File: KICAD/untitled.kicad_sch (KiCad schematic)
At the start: 46 parts, among them IC1 TPA3116D2QDADRQ1, U5 LM321

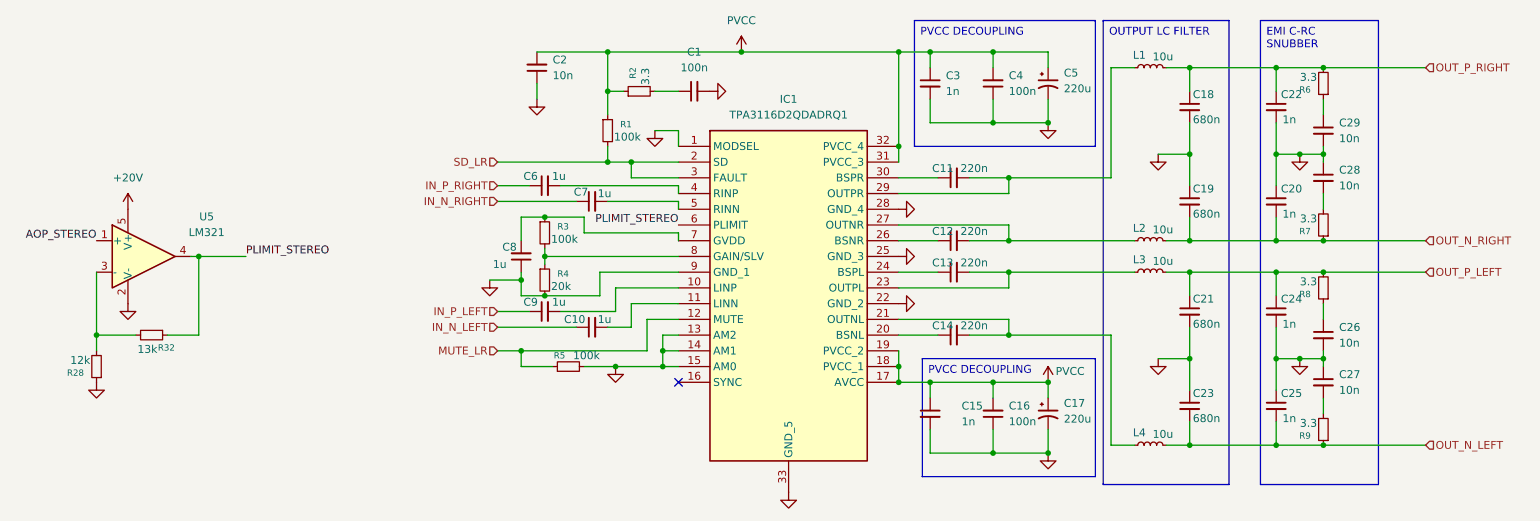
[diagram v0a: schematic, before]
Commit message: mise en forme globale
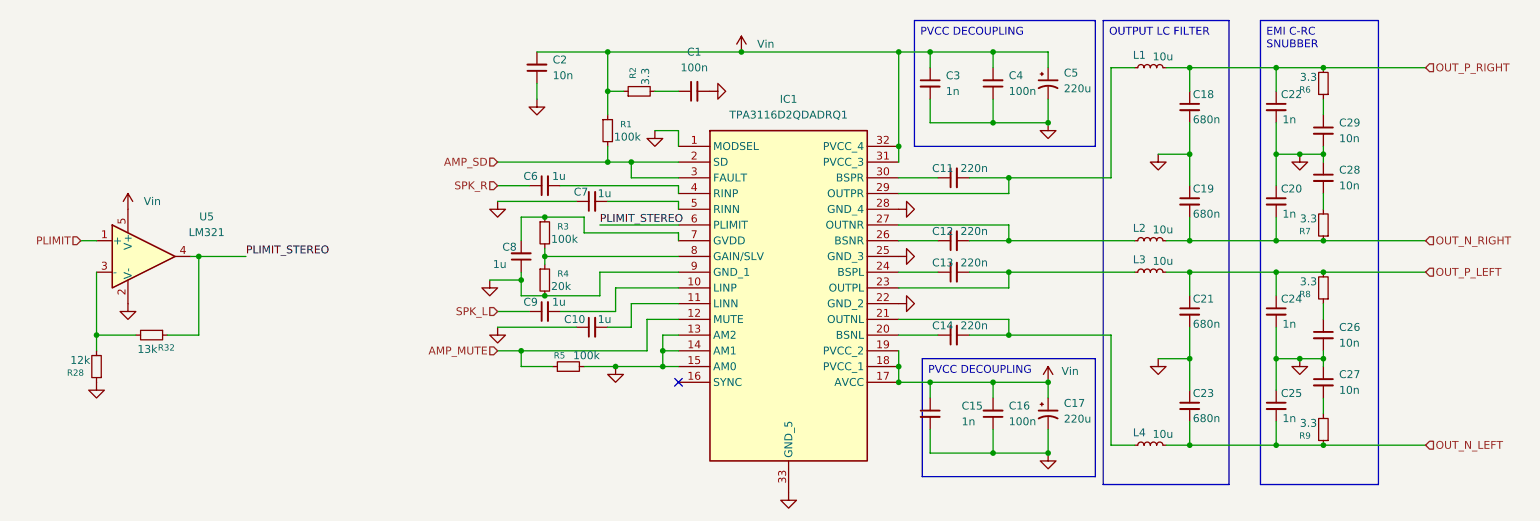
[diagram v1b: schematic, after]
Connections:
- net IN_N_LEFT is gone; now on net GND: C10.1
- net IN_N_RIGHT is gone; now on net GND: C7.1
- net PVCC is gone; now on net Vin: C15.1, C16.2, C17.1, C2.2, C3.1, C4.2, C5.1, IC1.17 (AVCC), IC1.18 (PVCC_1), IC1.19 (PVCC_2), IC1.31 (PVCC_3), IC1.32 (PVCC_4), R1.1, R2.1
- net +20V renamed Vin
- net AOP_STEREO renamed PLIMIT
- net IN_P_LEFT renamed SPK_L
- net IN_P_RIGHT renamed SPK_R
- net MUTE_LR renamed AMP_MUTE
- net SD_LR renamed AMP_SD
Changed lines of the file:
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@@
 	(wire
 		(pts
+			(xy 81.28 127) (xy 83.82 127)
+		)
+		(stroke
+			(width 0)
+			(type default)
+		)
+	)
+	(wire
+		(pts
 			(xy 281.94 119.38) (xy 281.94 121.92)
 		)
@@
 	(wire
 		(pts
+			(xy 165.1 124.46) (xy 177.8 124.46)
+		)
+		(stroke
+			(width 0)
+			(type default)
+		)
+	)
+	(wire
+		(pts
 			(xy 156.21 123.19) (xy 162.56 123.19)
 		)
@@
 		)
 	)
-	(label "AOP_STEREO"
-		(at 83.82 127 180)
-		(effects
-			(font
-				(size 1.27 1.27)
-			)
-			(justify right bottom)
-		)
-	)
 	(label "PLIMIT_STEREO"
-		(at 177.8 124.46 180)
+		(at 165.1 124.46 0)
 		(effects
 			(font
 				(size 1.27 1.27)
 			)
-			(justify right bottom)
+			(justify left bottom)
 		)
 	)
@@
 		)
 	)
-	(hierarchical_label "SD_LR"
+	(hierarchical_label "AMP_SD"
 		(shape input)
 		(at 148.59 114.3 180)
@@
 		)
 	)
-	(hierarchical_label "IN_P_LEFT"
+	(hierarchical_label "SPK_L"
 		(shape input)
 		(at 148.59 138.43 180)
@@
 		)
 	)
-	(hierarchical_label "MUTE_LR"
+	(hierarchical_label "AMP_MUTE"
 		(shape input)
 		(at 148.59 144.78 180)
@@
 		)
 	)
-	(hierarchical_label "IN_P_RIGHT"
+	(hierarchical_label "SPK_R"
 		(shape input)
 		(at 148.59 118.11 180)
@@
 		)
 	)
-	(hierarchical_label "IN_N_LEFT"
-		(shape input)
-		(at 148.59 140.97 180)
-		(effects
-			(font
-				(size 1.27 1.27)
-			)
-			(justify right)
-		)
-	)
 	(hierarchical_label "OUT_P_RIGHT"
 		(shape input)
@@
 		)
 	)
-	(hierarchical_label "IN_N_RIGHT"
+	(hierarchical_label "PLIMIT"
 		(shape input)
-		(at 148.59 120.65 180)
+		(at 81.28 127 180)
 		(effects
 			(font
@@
 			)
 		)
-		(property "Value" "PVCC"
-			(at 187.96 91.44 0)
+		(property "Value" "Vin"
+			(at 190.5 95.2499 0)
 			(show_name no)
 			(do_not_autoplace no)
@@
 					(size 1.27 1.27)
 				)
+				(justify left)
 			)
 		)
@@
 			)
 		)
-		(property "Value" "PVCC"
+		(property "Value" "Vin"
 			(at 241.046 148.082 0)
 			(show_name no)
@@
 	)
 	(symbol
+		(lib_id "power:GND")
+		(at 148.59 120.65 0)
+		(unit 1)
+		(body_style 1)
+		(exclude_from_sim no)
+		(in_bom yes)
+		(on_board yes)
+		(in_pos_files yes)
+		(dnp no)
+		(fields_autoplaced yes)
+		(property "Reference" "#PWR018"
+			(at 148.59 127 0)
+			(hide yes)
+			(show_name no)
+			(do_not_autoplace no)
+			(effects
+				(font
+					(size 1.27 1.27)
+				)
+			)
+		)
+		(property "Value" "GND"
+			(at 148.59 125.73 0)
+			(hide yes)
+			(show_name no)
+			(do_not_autoplace no)
+			(effects
+				(font
+					(size 1.27 1.27)
+				)
+			)
+		)
+		(property "Footprint" ""
+			(at 148.59 120.65 0)
+			(hide yes)
+			(show_name no)
+			(do_not_autoplace no)
+			(effects
+				(font
+					(size 1.27 1.27)
+				)
+			)
+		)
+		(property "Datasheet" ""
+			(at 148.59 120.65 0)
+			(hide yes)
+			(show_name no)
+			(do_not_autoplace no)
+			(effects
+				(font
+					(size 1.27 1.27)
+				)
+			)
+		)
+		(property "Description" "Power symbol creates a global label with name \"GND\" , ground"
+			(at 148.59 120.65 0)
+			(hide yes)
+			(show_name no)
+			(do_not_autoplace no)
+			(effects
+				(font
+					(size 1.27 1.27)
+				)
+			)
+		)
+		(pin "1"
+		)
+		(instances
+			(project "projet_2A"
+				(path "/05601714-c31e-4eda-914b-0c4b098c219a/d2c03650-eb6b-438f-8291-6b9088b7ba31"
+					(reference "#PWR018")
+					(unit 1)
+				)
+			)
+		)
+	)
+	(symbol
 		(lib_id "Device:R_Small")
 		(at 156.21 133.35 0)
@@
 			)
 		)
-		(property "Value" "+20V"
-			(at 88.9 116.84 0)
+		(property "Value" "Vin"
+			(at 91.44 120.6499 0)
 			(show_name no)
 			(do_not_autoplace no)
@@
 					(size 1.27 1.27)
 				)
+				(justify left)
 			)
 		)
@@
 					(unit 1)
 				)
+			)
+		)
+	)
+	(symbol
+		(lib_id "power:GND")
+		(at 148.59 140.97 0)
+		(unit 1)
+		(body_style 1)
+		(exclude_from_sim no)
+		(in_bom yes)
+		(on_board yes)
+		(in_pos_files yes)
+		(dnp no)
+		(fields_autoplaced yes)
+		(property "Reference" "#PWR019"
+			(at 148.59 147.32 0)
+			(hide yes)
+			(show_name no)
+			(do_not_autoplace no)
+			(effects
+				(font
+					(size 1.27 1.27)
+				)
+			)
+		)
+		(property "Value" "GND"
+			(at 148.59 146.05 0)
+			(hide yes)
+			(show_name no)
+			(do_not_autoplace no)
+			(effects
+				(font
+					(size 1.27 1.27)
+				)
+			)
+		)
+		(property "Footprint" ""
+			(at 148.59 140.97 0)
+			(hide yes)
+			(show_name no)
+			(do_not_autoplace no)
+			(effects
+				(font
+					(size 1.27 1.27)
+				)
+			)
+		)
+		(property "Datasheet" ""
+			(at 148.59 140.97 0)
+			(hide yes)
+			(show_name no)
+			(do_not_autoplace no)
+			(effects
+				(font
+					(size 1.27 1.27)
+				)
+			)
+		)
+		(property "Description" "Power symbol creates a global label with name \"GND\" , ground"
+			(at 148.59 140.97 0)
+			(hide yes)
+			(show_name no)
+			(do_not_autoplace no)
+			(effects
+				(font
+					(size 1.27 1.27)
+				)
+			)
+		)
+		(pin "1"
+		)
+		(instances
+			(project "projet_2A"
+				(path "/05601714-c31e-4eda-914b-0c4b098c219a/d2c03650-eb6b-438f-8291-6b9088b7ba31"
+					(reference "#PWR019")
+					(unit 1)
+				)
